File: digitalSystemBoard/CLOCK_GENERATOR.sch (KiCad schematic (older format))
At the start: 45 parts, among them J12 USB_OTG, Q22 Q_PMOS_GSD, SW4 ButtonFirst, SW5 ButtonFirst, SW6 ButtonFirst, SW7 ButtonFirst, U17 Potentiometer-digitalSystemBo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, U18 ICSP, U19 LP2985-3.3, U3 ATmega32U4-AU, U4 LMV358IDGKR, Y1 16MHz

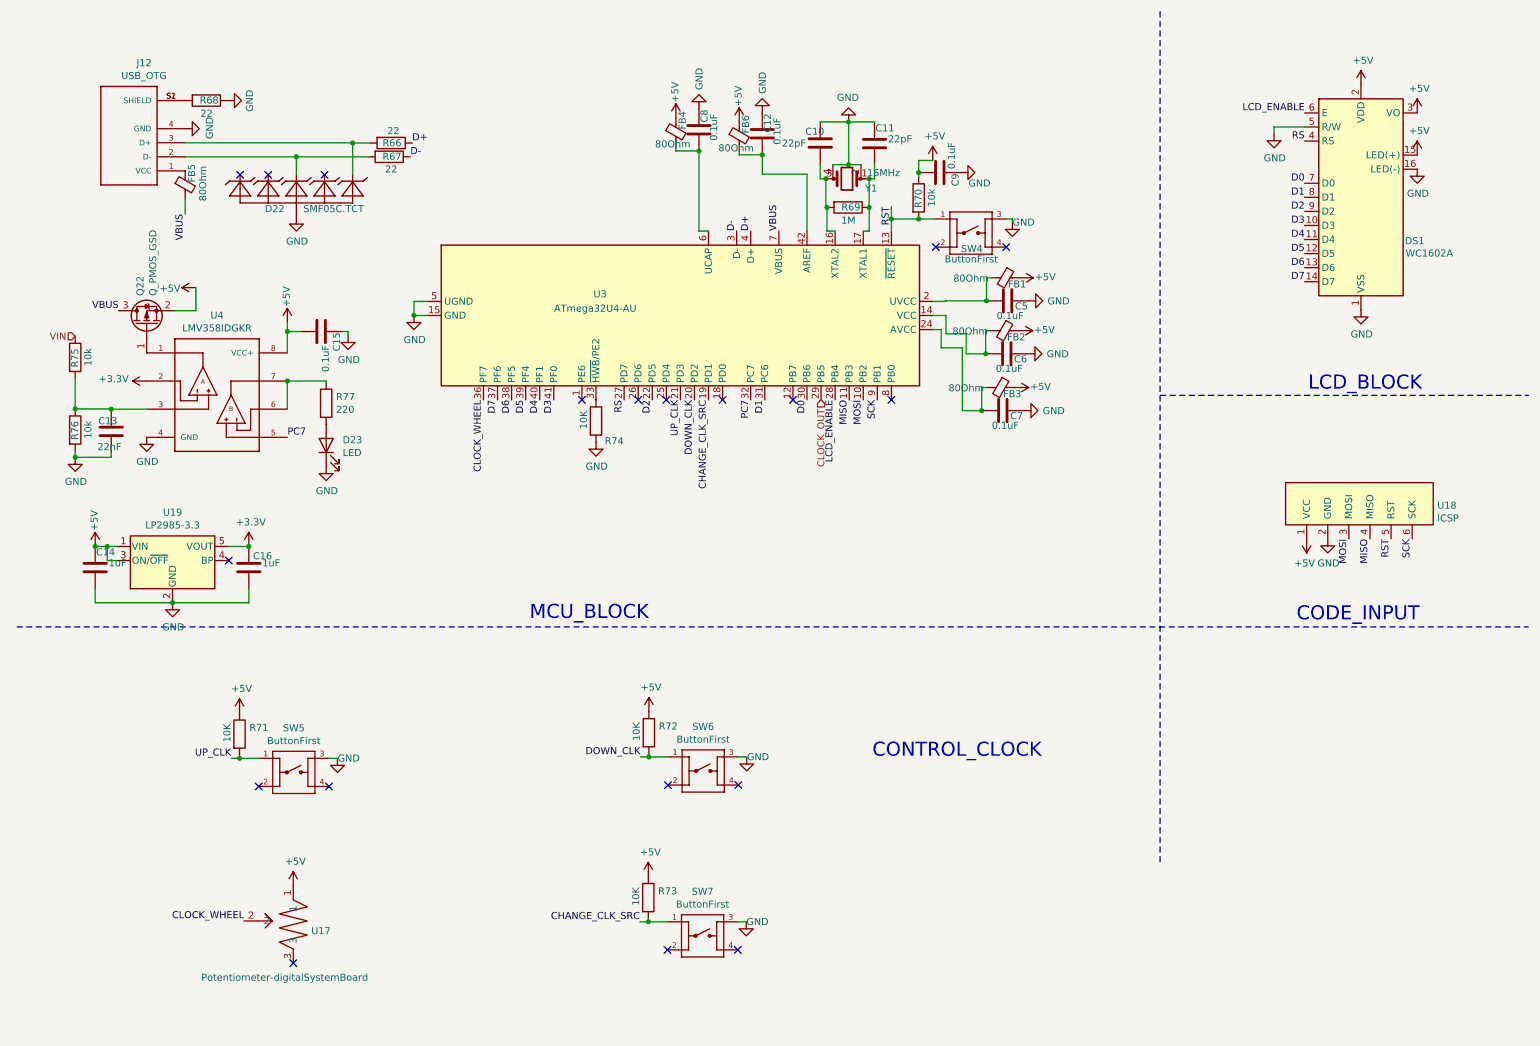
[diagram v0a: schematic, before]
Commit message: Update I/O and MCU schematic
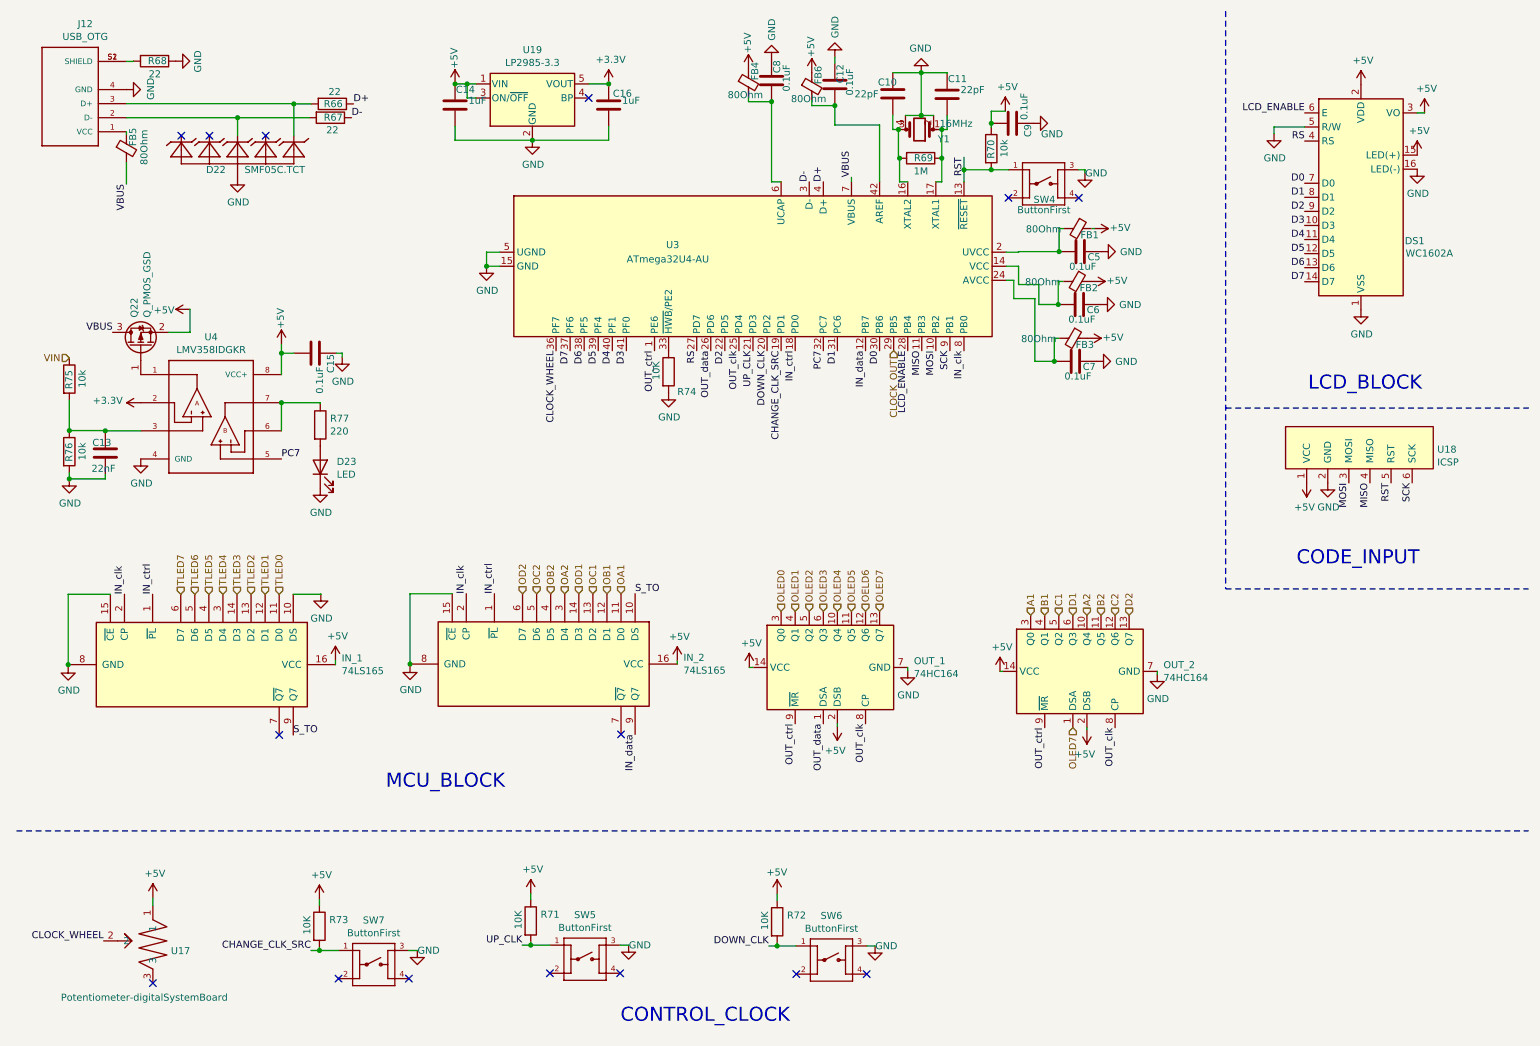
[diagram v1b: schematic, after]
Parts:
- added IN_1, IN_2: 74LS165, symbol 74xx:74LS165
- added OUT_1, OUT_2: 74HC164, symbol 74xx:74HC164
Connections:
- net +5V: now also IN_1.16 (VCC), IN_2.16 (VCC), OUT_1.14 (VCC), OUT_1.2 (DSB), OUT_2.14 (VCC), OUT_2.2 (DSB)
- net D1: now also OUT_2.6 (Q3)
- net D2: now also OUT_2.13 (Q7)
- net GND: now also IN_1.10 (DS), IN_1.15 (~CE), IN_1.8 (GND), IN_2.15 (~CE), IN_2.8 (GND), OUT_1.7 (GND), OUT_2.7 (GND)
- net OUT_ctrl: now reaches U3.1 (PE6)
- net OUT_ctrl: now also OUT_1.9 (~MR), OUT_2.9 (~MR)
- net IN_data: now reaches U3.12 (PB7)
- net IN_data: now also IN_2.9 (Q7)
- net IN_ctrl: now reaches U3.18 (PD0)
- net IN_ctrl: now also IN_1.1 (~PL), IN_2.1 (~PL)
- net OUT_clk: now reaches U3.25 (PD4)
- net OUT_clk: now also OUT_1.8 (CP), OUT_2.8 (CP)
- net OUT_data: now reaches U3.26 (PD6)
- net OUT_data: now also OUT_1.1 (DSA)
- net IN_clk: now reaches U3.8 (PB0)
- net IN_clk: now also IN_1.2 (CP), IN_2.2 (CP)
- new net A1: OUT_2.3 (Q0)
- new net A2: OUT_2.10 (Q4)
- new net B1: OUT_2.4 (Q1)
- new net B2: OUT_2.11 (Q5)
- new net C1: OUT_2.5 (Q2)
- new net C2: OUT_2.12 (Q6)
- new net OA1: IN_2.11 (D0)
- new net OA2: IN_2.3 (D4)
- new net OB1: IN_2.12 (D1)
- new net OB2: IN_2.4 (D5)
- new net OC1: IN_2.13 (D2)
- new net OC2: IN_2.5 (D6)
- new net OD1: IN_2.14 (D3)
- new net OD2: IN_2.6 (D7)
- new net OELD6: OUT_1.12 (Q6)
- new net OLED0: OUT_1.3 (Q0)
- new net OLED1: OUT_1.4 (Q1)
- new net OLED2: OUT_1.5 (Q2)
- new net OLED3: OUT_1.6 (Q3)
- new net OLED4: OUT_1.10 (Q4)
- new net OLED5: OUT_1.11 (Q5)
- new net OLED7: OUT_1.13 (Q7), OUT_2.1 (DSA)
- new net S_TO: IN_1.9 (Q7), IN_2.10 (DS)
- new net TLED0: IN_1.11 (D0)
- new net TLED1: IN_1.12 (D1)
- new net TLED2: IN_1.13 (D2)
- new net TLED3: IN_1.14 (D3)
- new net TLED4: IN_1.3 (D4)
- new net TLED5: IN_1.4 (D5)
- new net TLED6: IN_1.5 (D6)
- new net TLED7: IN_1.6 (D7)
- no-connect marks 19 -> 15
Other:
- moved on the sheet: C10, C11, C12, C13, C14, C15, C16, C5, C6, C7, C8, C9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

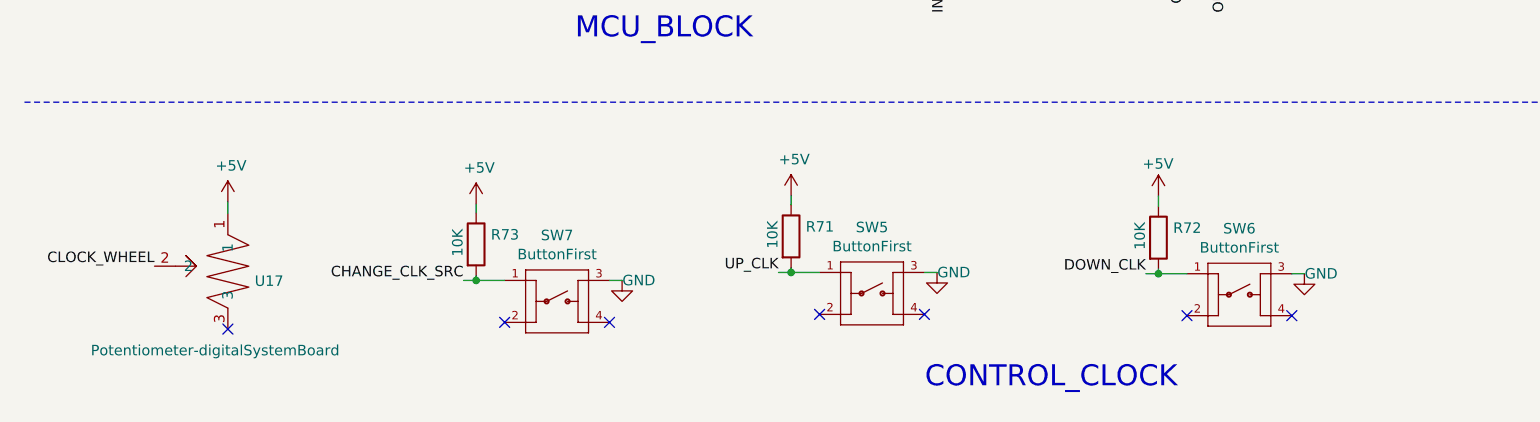
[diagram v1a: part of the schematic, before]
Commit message: Update I/O schematic, Complete layout, Start routing
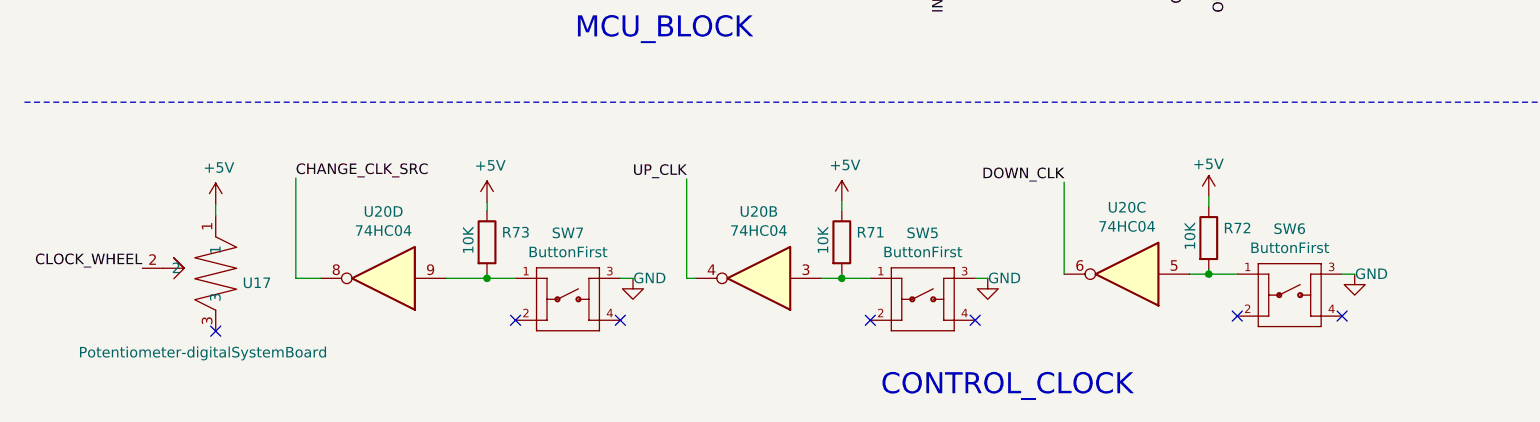
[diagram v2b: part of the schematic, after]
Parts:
- added U20: 74HC04, symbol 74xx:74HC04
- IN_1, IN_2: footprint (none) -> Package_SO:SOIC-16_3.9x9.9mm_P1.27mm
- OUT_1, OUT_2: footprint (none) -> Package_SO:SOIC-14_3.9x8.7mm_P1.27mm
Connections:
- net CHANGE_CLK_SRC: now also U20.8; no longer R73.2, SW7.1
- net DOWN_CLK: now also U20.6; no longer R72.2, SW6.1
- net UP_CLK: now also U20.4; no longer R71.2, SW5.1
- new net: R72.2, SW6.1, U20.5
- new net: R71.2, SW5.1, U20.3
- new net: R73.2, SW7.1, U20.9
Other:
- moved on the sheet: R71, R72, R73, SW5, SW6, SW7, U17
